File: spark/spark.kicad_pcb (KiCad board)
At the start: 2 copper layers, 49.7 x 56.8 mm, 37 parts, among them J1 USB_B_Mini, J2 Screw_Terminal_01x03, K1 SRD-03VDC-SL-C, Q1 SS8050-G, Q2 SS8050-G, Q3 2N3904, SW1/BOOT1 SW_Push, SW2/EN1 SW_Push, U1 AMS1117-3.3, U2 CP2102N-Axx-xQFN28, U3 ESP32-WROOM-32

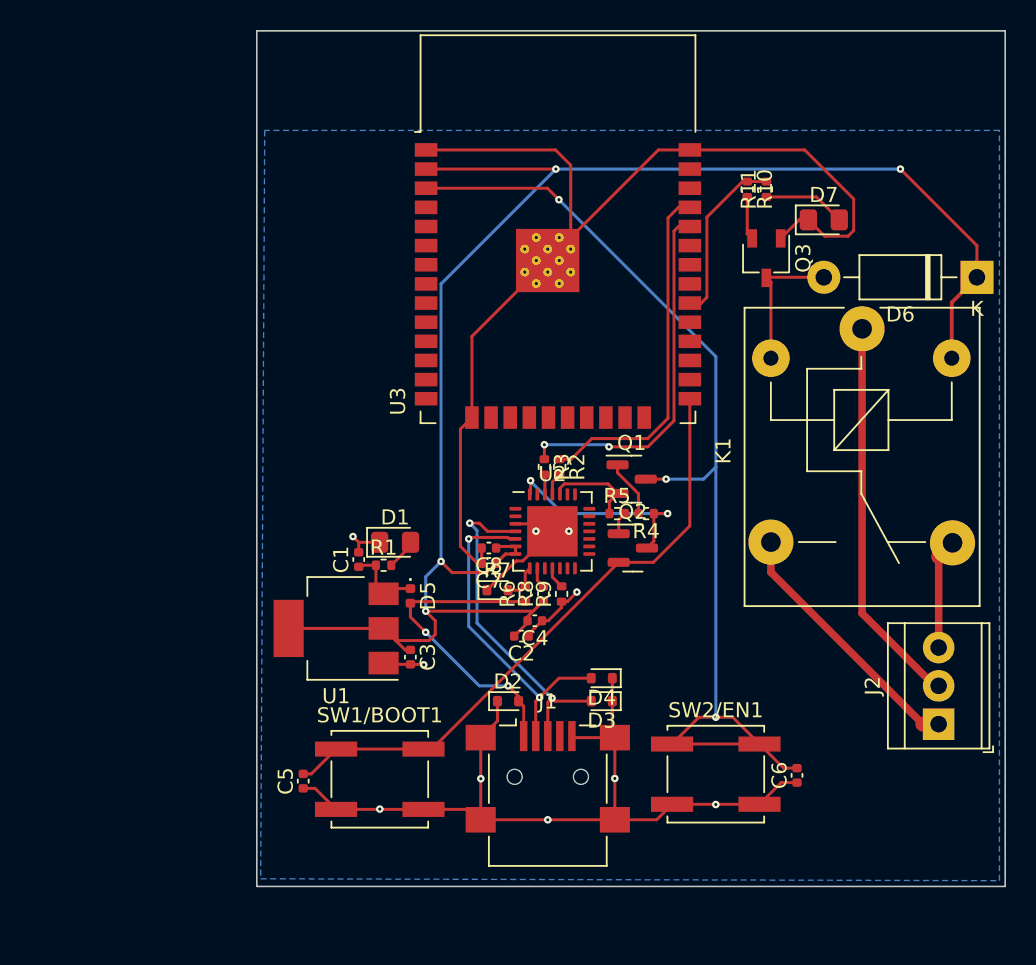
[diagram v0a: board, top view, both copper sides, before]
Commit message: Another checkpoint, going to do layout again for funsies
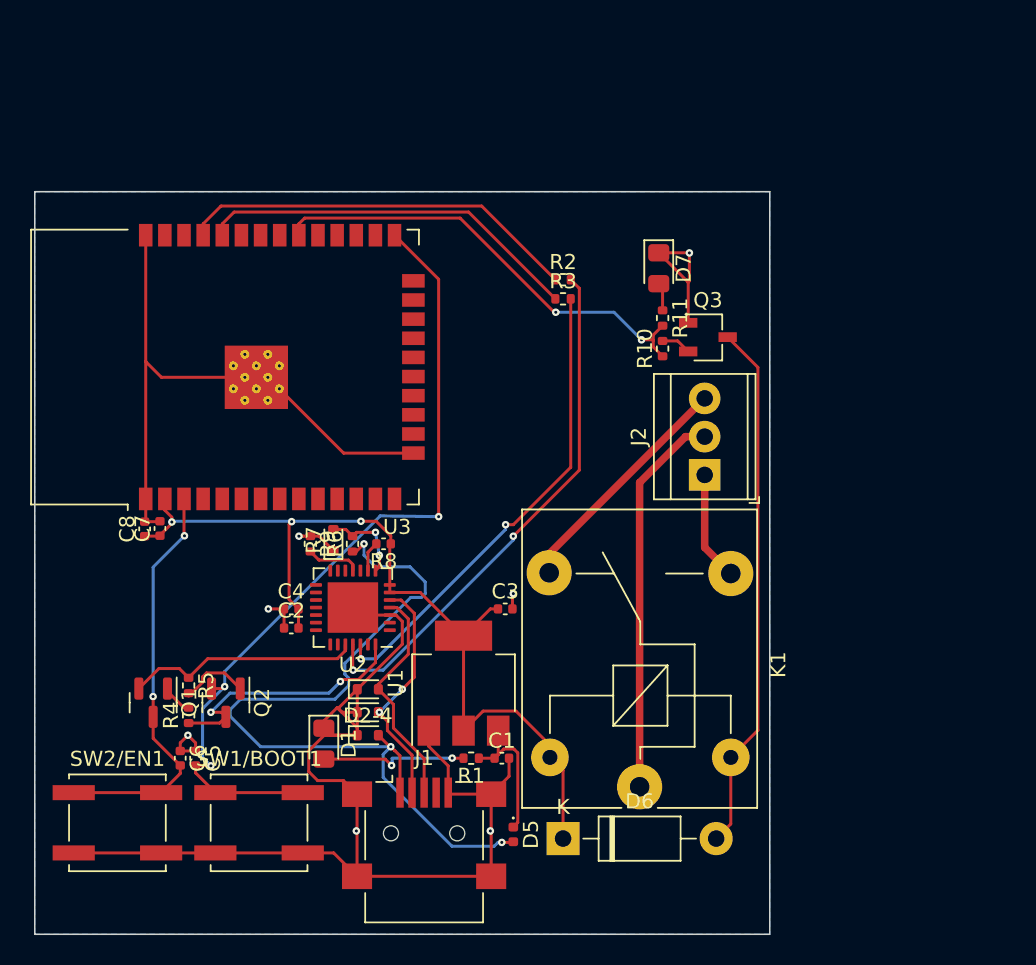
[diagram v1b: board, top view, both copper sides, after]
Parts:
- removed D2: ESD5Zxx, Diode_SMD:D_SOD-523
- added D2-4: ESD5Zxx, Diode_SMD:D_SOD-523, F.Cu at (99.8, 111.8)
- moved D6 46.3 mm to (112.8, 118.6), turned to 0 degrees
- moved C6 40.9 mm to (87.4, 113.3), turned to -90 degrees
- moved SW2/EN1 39.8 mm to (83.2, 117.6)
- moved Q1 35.0 mm to (85.6, 109.6), turned to -90 degrees
- moved K1 33.8 mm to (117.9, 115.2), turned to 90 degrees
- moved R4 33.2 mm to (87.9, 110.4), turned to 90 degrees
- moved R5 30.6 mm to (87.9, 108.5), turned to -90 degrees
- moved Q2 28.9 mm to (90.4, 109.6), turned to -90 degrees
- moved C8 22.9 mm to (85.0, 98.1), turned to 90 degrees
- moved J2 22.7 mm to (122.2, 94.5)
- moved C7 21.9 mm to (86.0, 98.0), turned to 90 degrees
- moved U3 20.1 mm to (93.3, 87.3), turned to 90 degrees
- moved D5 17.2 mm to (109.5, 118.3)
- moved R9 17.0 mm to (96.0, 99.1), turned to -90 degrees
- moved C1 16.2 mm to (108.7, 113.3), turned to 0 degrees
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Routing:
- net VDD33: track 111.7 -> 59.4 mm, vias 4 -> 3
- net EN: track 69.0 -> 27.4 mm, vias 3 -> 2
- net RXD: track 1.52 -> 35.2 mm, vias 0 -> 2
- net VBUS: track 20.7 -> 53.9 mm, vias 2 -> 3
- net TXD: track 1.33 -> 31.5 mm, vias 0 -> 2
- net Net-(D6-A): track 9.28 -> 35.3 mm
- net IO18: track 11.5 -> 30.4 mm, vias 0 -> 2
- net IO0: track 40.9 -> 55.7 mm, vias 0 -> 3
- net R1N0: track 17.3 -> 7.26 mm
- net RTS: track 6.18 -> 15.7 mm
- net R1NC: track 7.33 -> 15.8 mm
- net Net-(D1-A): track 2.05 -> 10.1 mm, vias 0 -> 2
- net USB_DP: track 22.5 -> 15.5 mm, vias 2 -> 0
- net GND: track 148.0 -> 141.3 mm, vias 10 -> 7
- net USB_DN: track 22.3 -> 15.8 mm
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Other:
- board size 49.7 x 56.8 mm -> 48.8 x 49.3 mm
